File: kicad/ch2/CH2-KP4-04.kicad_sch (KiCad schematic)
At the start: 7 parts

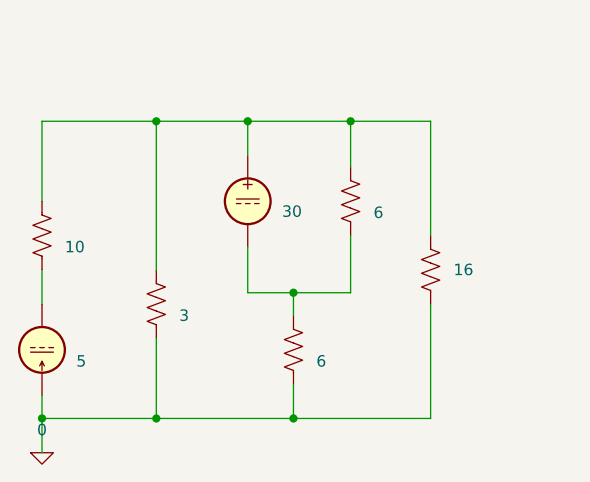
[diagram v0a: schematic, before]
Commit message: regular
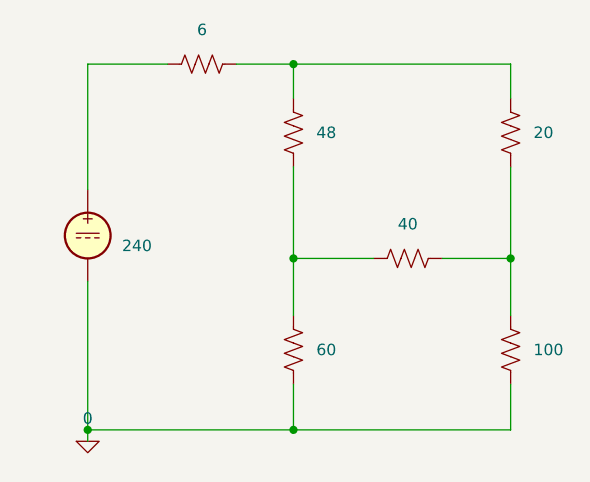
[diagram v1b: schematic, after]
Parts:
- removed I6: 5, symbol Simulation_SPICE:IDC
- removed R29: 10, symbol Device:R_US
- removed R30: 3, symbol Device:R_US
- removed R31, R32: 6, symbol Device:R_US
- removed R33: 16, symbol Device:R_US
- removed V12: 30, symbol Simulation_SPICE:VDC
- added R46: 48, symbol Device:R_US
- added R47: 20, symbol Device:R_US
- added R48: 60, symbol Device:R_US
- added R49: 100, symbol Device:R_US
- added R50: 40, symbol Device:R_US
- added R51: 6, symbol Device:R_US
- added V17: 240, symbol Simulation_SPICE:VDC
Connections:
- net 0: now also R48.1, R49.1, V17.2
- new net: R46.1, R48.2, R50.2
- new net: R46.2, R47.2, R51.1
- new net: R51.2, V17.1
- new net: R47.1, R49.2, R50.1
